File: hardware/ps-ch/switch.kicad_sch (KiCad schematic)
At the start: 11 parts, among them Q4 PSMN059-150Y, Q9 PSMN059-150Y, U16 LM74502H

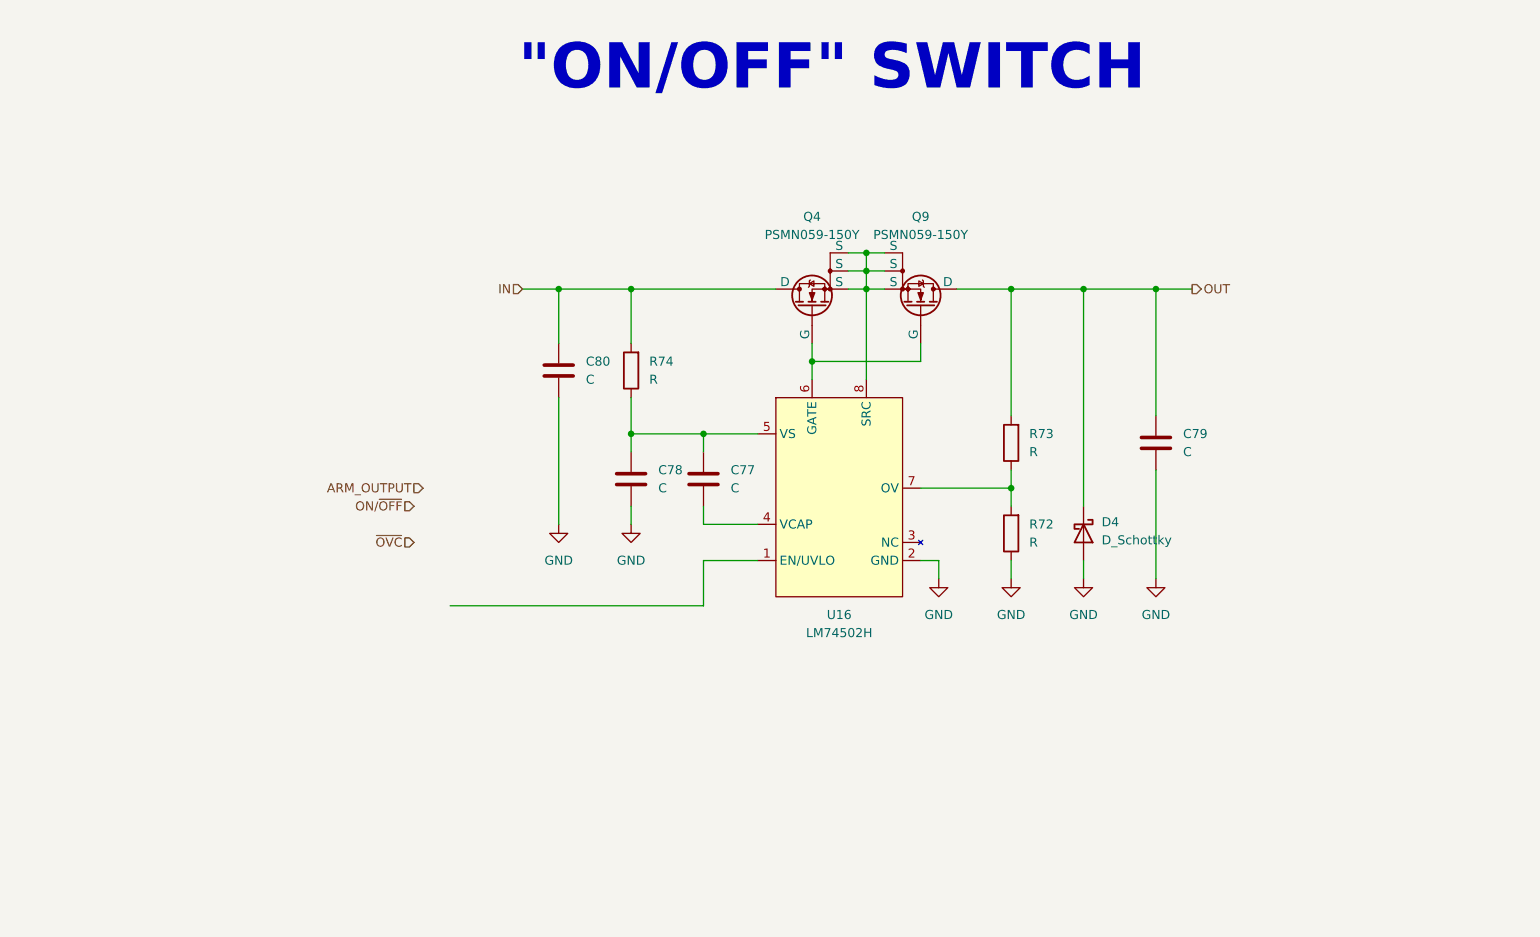
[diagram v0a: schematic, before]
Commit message: drawn enabled circuit
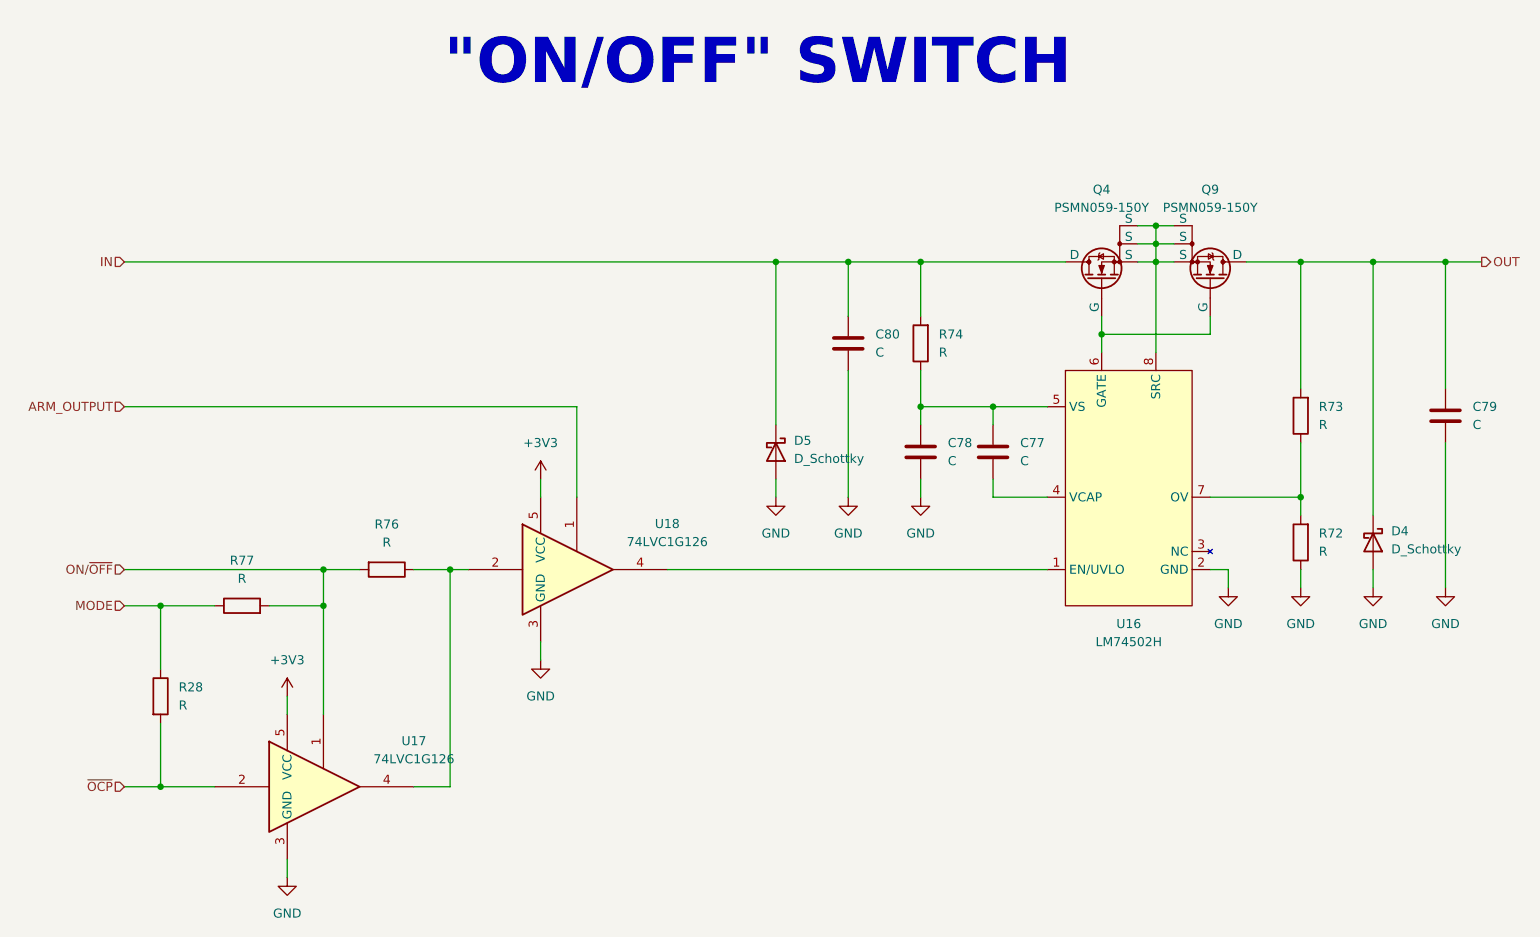
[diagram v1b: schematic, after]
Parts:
- added D5: D_Schottky, symbol Device:D_Schottky
- added R28, R76, R77: R, symbol Device:R
- added U17, U18: 74LVC1G126, symbol 74xGxx:74LVC1G126
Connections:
- net ARM_OUTPUT: now also U18.1
- net GND: now also D5.2 (A), U17.3 (GND), U18.3 (GND)
- net IN: now also D5.1 (K)
- net ON/~{OFF}: now also R76.2, R77.2, U17.1
- net at U16.1 (EN/UVLO): now also U18.4
- new net: R76.1, U17.4, U18.2
- new net +3V3: U17.5 (VCC), U18.5 (VCC)
- new net MODE: R28.1, R77.1
- new net ~{OCP}: R28.2, U17.2
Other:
- moved on the sheet: C77, C78, C79, C80, D4, Q4, Q9, R72, R73, R74, U16
